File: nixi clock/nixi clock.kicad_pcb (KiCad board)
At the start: 2 copper layers, 16 parts, among them IC1 ESP32-S3-WROOM-1U-N4, IC2 74AHCT595PW-Q100,1, IC3 74AHCT595PW-Q100,1, IC4 PCF85063AT_AY, IC5 74141, IC6 74141, IC7 74141, IC8 74141, IC9 LM1117MP-3.3_NOPB

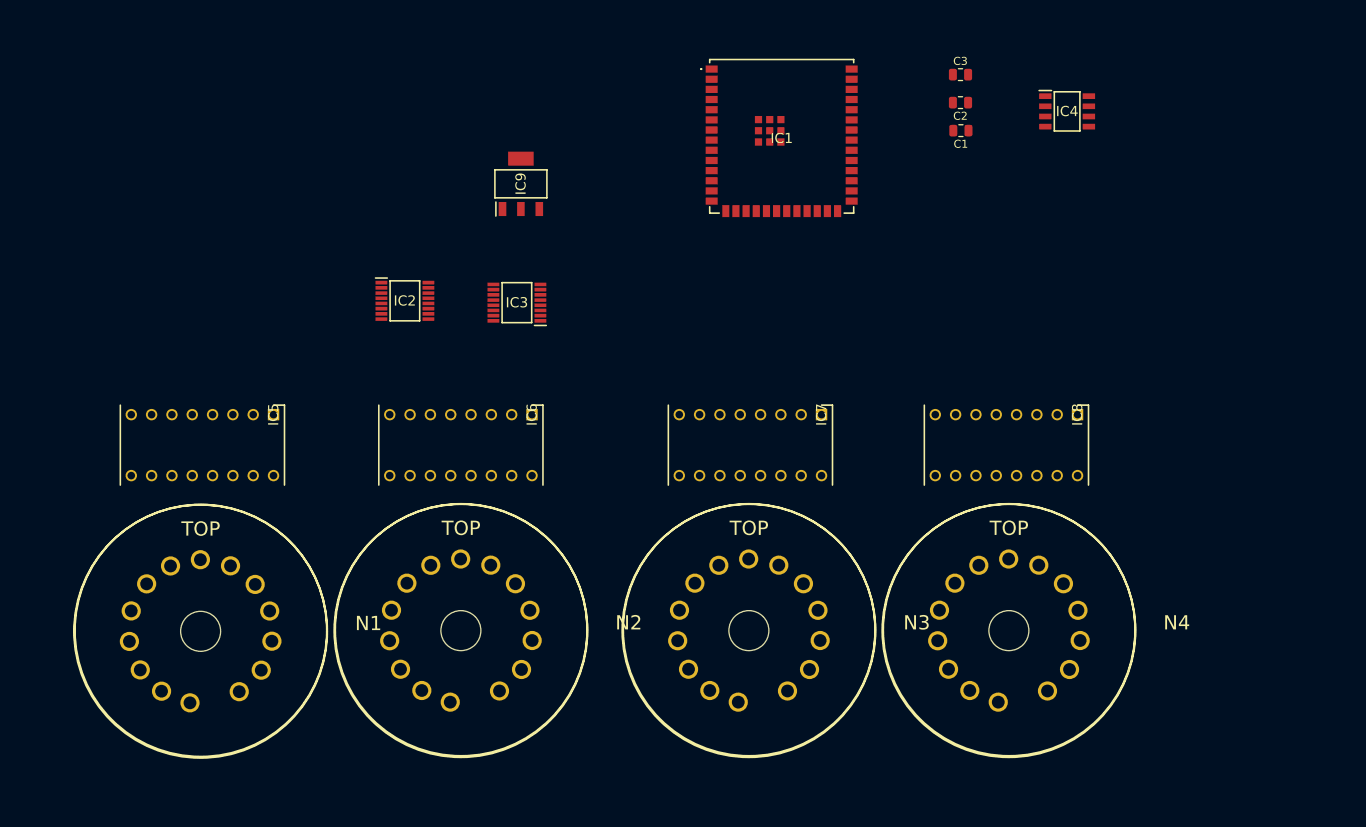
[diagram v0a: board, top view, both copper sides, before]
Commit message: nixi clock
first pcb version
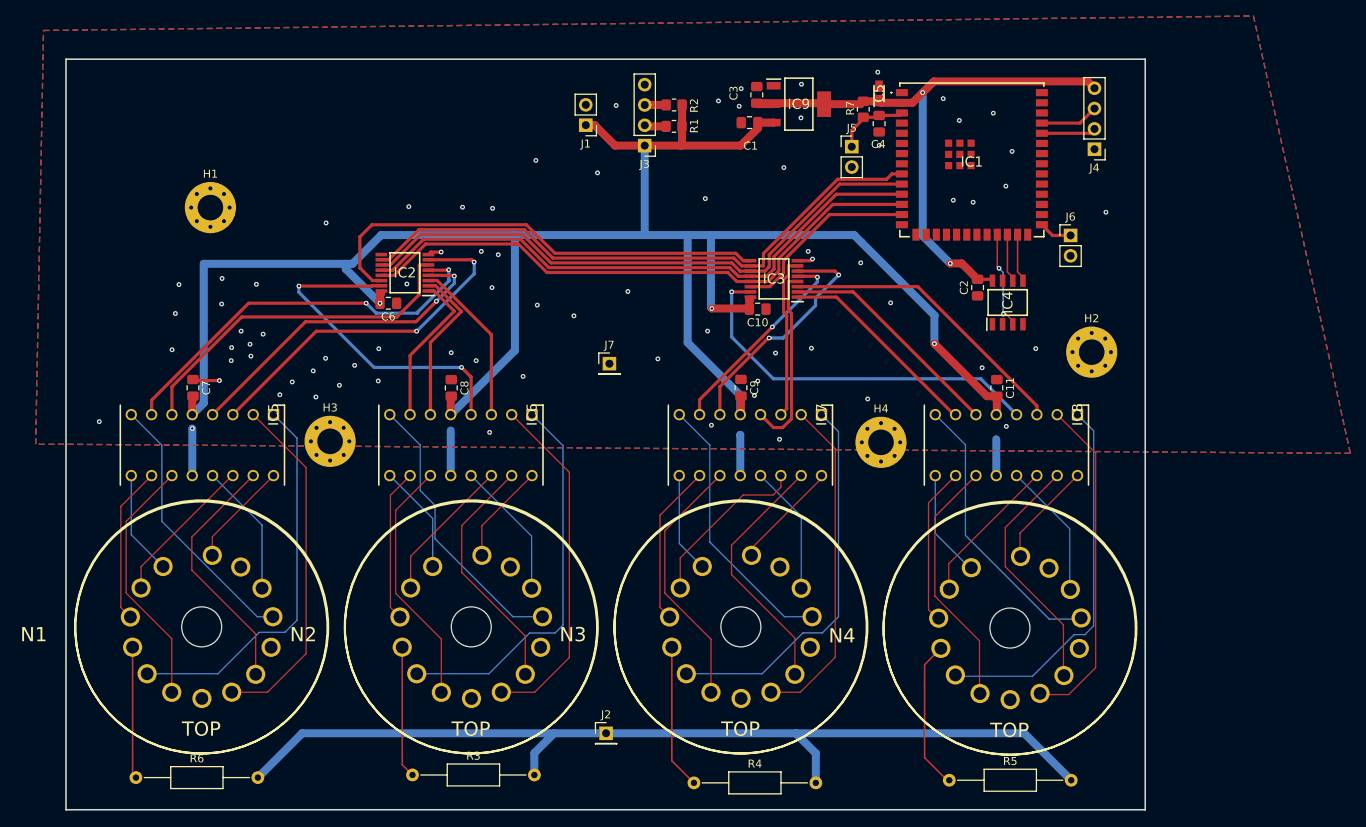
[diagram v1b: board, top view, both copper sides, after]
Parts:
- added C10: 10u, Capacitor_SMD:C_0805_2012Metric_Pad1.18x1.45mm_HandSolder, F.Cu at (204.6, 95.8)
- added C11: 10u, Capacitor_SMD:C_0805_2012Metric_Pad1.18x1.45mm_HandSolder, F.Cu at (234.5, 105.7)
- added C4: 10u, Capacitor_SMD:C_0805_2012Metric_Pad1.18x1.45mm_HandSolder, F.Cu at (219.8, 72.6)
- added C5: TMCP0G476MTR2F, SamacSys_Parts:CAPPM2012X120N, F.Cu at (219.8, 68.8)
- added C6: 10u, Capacitor_SMD:C_0805_2012Metric_Pad1.18x1.45mm_HandSolder, F.Cu at (158.4, 95.1)
- added C7: 10u, Capacitor_SMD:C_0805_2012Metric_Pad1.18x1.45mm_HandSolder, F.Cu at (134.0, 105.7)
- added C8: 10u, Capacitor_SMD:C_0805_2012Metric_Pad1.18x1.45mm_HandSolder, F.Cu at (166.3, 105.7)
- added C9: 10u, Capacitor_SMD:C_0805_2012Metric_Pad1.18x1.45mm_HandSolder, F.Cu at (202.5, 105.6)
- added H1: MountingHole_Pad, MountingHole:MountingHole_3.2mm_M3_Pad_Via, F.Cu at (136.2, 83.1)
- added H2: MountingHole_Pad, MountingHole:MountingHole_3.2mm_M3_Pad_Via, F.Cu at (246.3, 101.2)
- added H3: MountingHole_Pad, MountingHole:MountingHole_3.2mm_M3_Pad_Via, F.Cu at (151.2, 112.3)
- added H4: MountingHole_Pad, MountingHole:MountingHole_3.2mm_M3_Pad_Via, F.Cu at (220.0, 112.5)
- added J1: Conn_01x02, Connector_PinHeader_2.54mm:PinHeader_1x02_P2.54mm_Vertical, F.Cu at (183.1, 72.8)
- added J2: Conn_01x01, Connector_PinHeader_2.54mm:PinHeader_1x01_P2.54mm_Vertical, F.Cu at (185.6, 148.8)
- added J3: Conn_01x04, Connector_PinHeader_2.54mm:PinHeader_1x04_P2.54mm_Vertical, F.Cu at (190.5, 75.4)
- added J4: Conn_01x04, Connector_PinHeader_2.54mm:PinHeader_1x04_P2.54mm_Vertical, F.Cu at (246.7, 75.8)
- added J5: Conn_01x02, Connector_PinHeader_2.54mm:PinHeader_1x02_P2.54mm_Vertical, F.Cu at (216.4, 75.5)
- added J6: Conn_01x02, Connector_PinHeader_2.54mm:PinHeader_1x02_P2.54mm_Vertical, F.Cu at (243.7, 86.6)
- added J7: Conn_01x01, Connector_PinHeader_2.54mm:PinHeader_1x01_P2.54mm_Vertical, F.Cu at (186.1, 102.6)
- added R1: 4k7, Resistor_SMD:R_0805_2012Metric_Pad1.20x1.40mm_HandSolder, F.Cu at (194.1, 73.0)
- added R2: 4k7, Resistor_SMD:R_0805_2012Metric_Pad1.20x1.40mm_HandSolder, F.Cu at (194.2, 70.3)
- added R3: 6k8, Resistor_THT:R_Axial_DIN0207_L6.3mm_D2.5mm_P15.24mm_Horizontal, F.Cu at (161.4, 154.0)
- added R4: 6k8, Resistor_THT:R_Axial_DIN0207_L6.3mm_D2.5mm_P15.24mm_Horizontal, F.Cu at (196.6, 155.0)
- added R5: 6k8, Resistor_THT:R_Axial_DIN0207_L6.3mm_D2.5mm_P15.24mm_Horizontal, F.Cu at (228.6, 154.7)
- added R6: 6k8, Resistor_THT:R_Axial_DIN0207_L6.3mm_D2.5mm_P15.24mm_Horizontal, F.Cu at (126.9, 154.4)
- added R7: 10k, Resistor_SMD:R_0805_2012Metric_Pad1.20x1.40mm_HandSolder, F.Cu at (217.8, 70.8)
- C1, C2, C3: value C -> 10u; footprint Capacitor_SMD:C_0805_2012Metric -> Capacitor_SMD:C_0805_2012Metric_Pad1.18x1.45mm_HandSolder
- moved IC9 36.1 mm to (209.8, 70.2), turned to 0 degrees
- moved IC3 32.3 mm to (206.6, 92.0)
- moved C1 26.4 mm to (203.6, 72.5), turned to 0 degrees
- moved C3 25.6 mm to (204.5, 69.0), turned to -90 degrees
- moved IC4 25.0 mm to (235.8, 95.0), turned to 90 degrees
- moved IC1 24.0 mm to (231.4, 77.4)
- moved C2 23.2 mm to (232.1, 93.1), turned to 90 degrees
- moved IC2 3.51 mm to (160.5, 91.3), turned to 180 degrees
- moved N2 1.27 mm to (168.8, 135.6), turned to 180 degrees
- moved N3 1.11 mm to (202.5, 135.6), turned to 180 degrees
- moved N1 0.39 mm to (135.1, 135.6), turned to 180 degrees
- moved N4 0.16 mm to (236.1, 135.8), turned to 180 degrees
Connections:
- IC1 pad 10: unconnected-(IC1-IO17-Pad10) -> D_CLK
- IC1 pad 11: unconnected-(IC1-IO18-Pad11) -> O_CLK
- IC1 pad 12: unconnected-(IC1-IO8-Pad12) -> NIXI_EN
- IC1 pad 13: unconnected-(IC1-IO19-Pad13) -> NIXI_DATA
- IC1 pad 27: unconnected-(IC1-IO0-Pad27) -> BOOT
- IC1 pad 28: NIXI_DATA -> unconnected-(IC1-IO35-Pad28)
- IC1 pad 29: NIXI_EN -> unconnected-(IC1-IO36-Pad29)
- IC1 pad 3: unconnected-(IC1-EN-Pad3) -> EN
- IC1 pad 30: O_CLK -> unconnected-(IC1-IO37-Pad30)
- IC1 pad 31: D_CLK -> unconnected-(IC1-IO38-Pad31)
- IC1 pad 36: unconnected-(IC1-RXD0-Pad36) -> RXD
- IC1 pad 37: unconnected-(IC1-TXD0-Pad37) -> TXD
- IC1 pad 9: unconnected-(IC1-IO16-Pad9) -> RST
- IC2 pad 9: unconnected-(IC2-Q7S-Pad9) -> Net-(IC2-Q7S)
- IC5 pad 3: unconnected-(IC5-Pad3) -> N1A
- IC5 pad 4: N1C -> N1D
- IC5 pad 7: unconnected-(IC5-Pad7) -> N1C
- N1 pad A3: VBUS -> Net-(N1-A)
- N2 pad A3: VBUS -> Net-(N2-A)
- N3 pad A3: VBUS -> Net-(N3-A)
- N4 pad A3: VBUS -> Net-(N4-A)
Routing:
- net +5V: track 0.00 -> 256.6 mm, vias 0 -> 3
- net VBUS: track 0.00 -> 119.9 mm
- net +3.3V: track 0.00 -> 75.1 mm, vias 0 -> 2
- net RST: track 0.00 -> 74.2 mm
- net D_CLK: track 0.00 -> 74.0 mm
- net O_CLK: track 0.00 -> 73.7 mm
- net NIXI_EN: track 0.00 -> 73.5 mm
- net R1DO: track 0.00 -> 58.5 mm
- net N1C: track 0.00 -> 50.3 mm, vias 0 -> 2
- net N29: track 0.00 -> 48.7 mm
- net N19: track 0.00 -> 48.4 mm
- net N39: track 0.00 -> 48.1 mm
- net N4D: track 0.00 -> 47.6 mm, vias 0 -> 1
- net N49: track 0.00 -> 47.2 mm
- net N1A: track 0.00 -> 44.8 mm, vias 0 -> 2
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- added copper zone on B.Cu, net GND
- added copper zone on F.Cu, net GND
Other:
- board outline added: 134.9 x 93.8 mm
